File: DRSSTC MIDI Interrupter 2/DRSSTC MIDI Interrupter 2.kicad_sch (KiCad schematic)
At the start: 67 parts, among them CN2 HX25003-2WAP, Q1 8205A_C5370944, Q2 AO3401A_C347476, SW1 SW_Push, SW2 SW_Push, U1 ESP32-S3-WROOM-1, U10 TPS63802DLAR, U11 BQ27441DRZR-G1B, U2 BQ24072RGT, U3 DW01A, U4 TPS61023DRLR, U6 SRV05-4, U7 USBLC6-2P6, U8 TS3USB221ARSER, U9 TL331

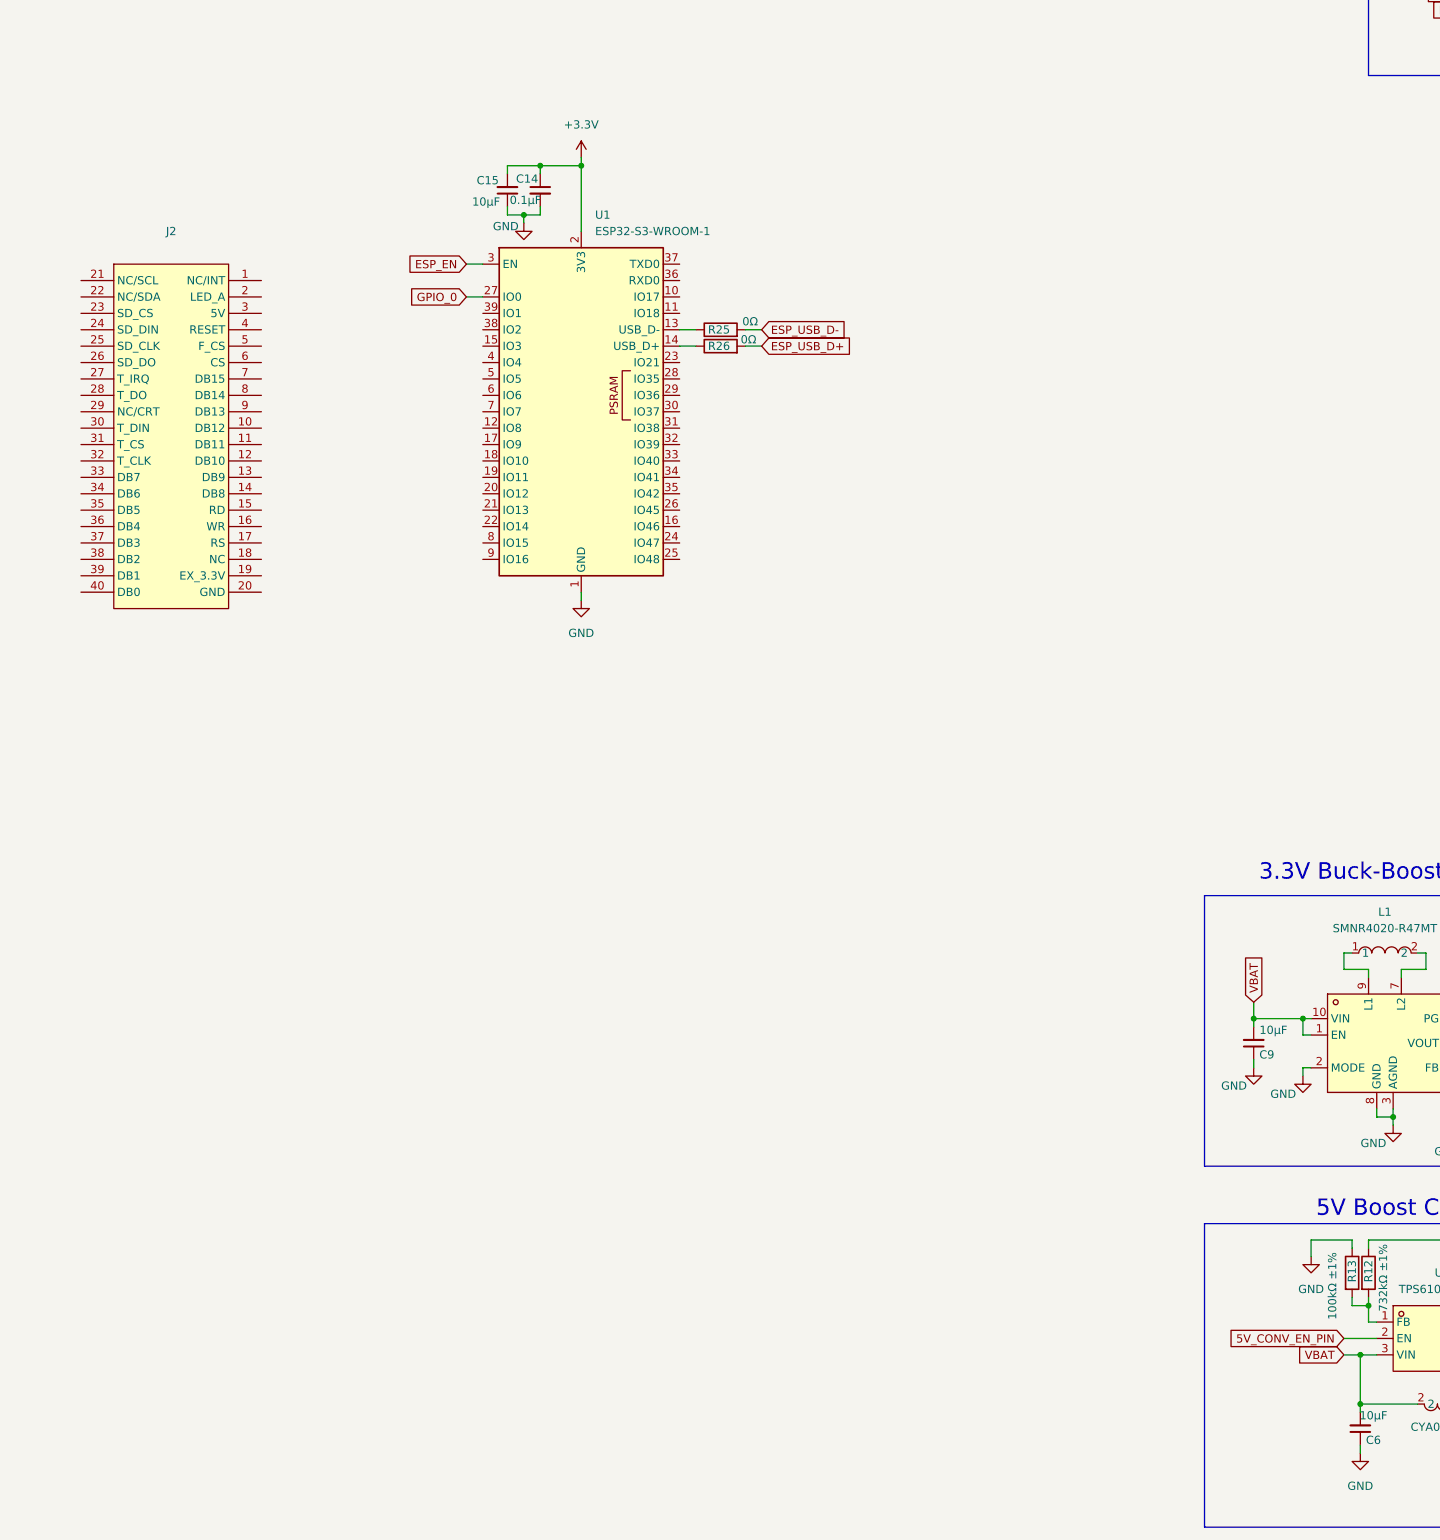
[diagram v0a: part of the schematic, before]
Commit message: Initial commit of components
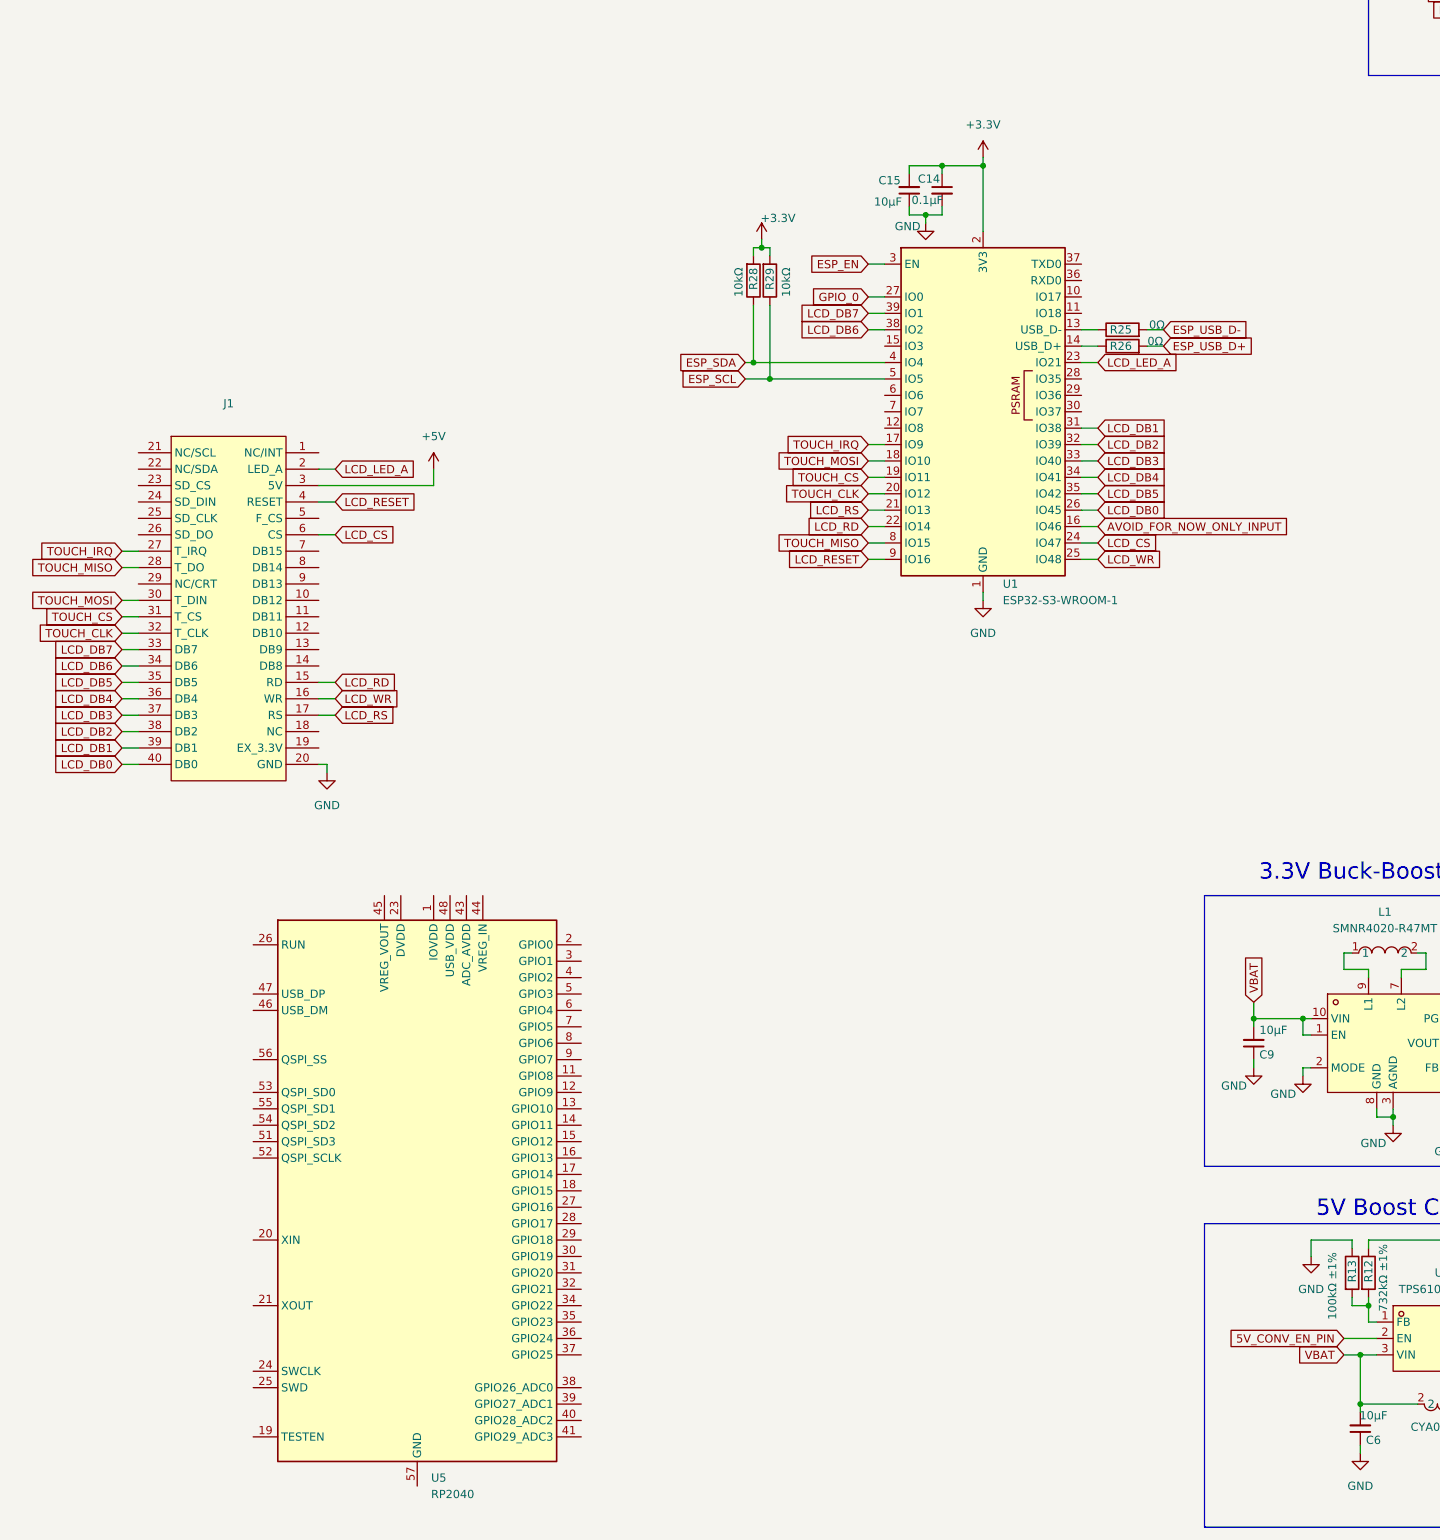
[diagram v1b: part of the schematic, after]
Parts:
- removed J2: ~, Custom Parts:LCD, symbol Custom Parts:LCD
- added J1: ~, parts:LCD, symbol parts:LCD
- added R28, R29: 10kΩ, Resistor_SMD:R_0805_2012Metric_Pad1.20x1.40mm_HandSolder, symbol Device:R
- added U5: RP2040, Package_DFN_QFN:QFN-56-1EP_7x7mm_P0.4mm_EP3.2x3.2mm, symbol MCU_RaspberryPi:RP2040
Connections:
- net +3.3V: now also R28.2, R29.2
- net +5V: now also J1.3 (5V)
- net ESP_SCL: now also U1.5 (IO5), R29.1
- net ESP_SDA: now also U1.4 (IO4), R28.1
- net GND: now also J1.20 (GND)
- net AVOID_FOR_NOW_ONLY_INPUT: now reaches U1.16 (IO46)
- net TOUCH_IRQ: now reaches U1.17 (IO9)
- net TOUCH_IRQ: now also J1.27 (T_IRQ)
- net TOUCH_MOSI: now reaches U1.18 (IO10)
- net TOUCH_MOSI: now also J1.30 (T_DIN)
- net TOUCH_CS: now reaches U1.19 (IO11)
- net TOUCH_CS: now also J1.31 (T_CS)
- net TOUCH_CLK: now reaches U1.20 (IO12)
- net TOUCH_CLK: now also J1.32 (T_CLK)
- net LCD_RS: now reaches U1.21 (IO13)
- net LCD_RS: now also J1.17 (RS)
- net LCD_RD: now reaches U1.22 (IO14)
- net LCD_RD: now also J1.15 (RD)
- net LCD_LED_A: now reaches U1.23 (IO21)
- net LCD_LED_A: now also J1.2 (LED_A)
- net LCD_CS: now reaches U1.24 (IO47)
- net LCD_CS: now also J1.6 (CS)
- net LCD_WR: now reaches U1.25 (IO48)
- net LCD_WR: now also J1.16 (WR)
- net LCD_DB0: now reaches U1.26 (IO45)
- net LCD_DB0: now also J1.40 (DB0)
- net LCD_DB1: now reaches U1.31 (IO38)
- net LCD_DB1: now also J1.39 (DB1)
- net LCD_DB2: now reaches U1.32 (IO39)
- net LCD_DB2: now also J1.38 (DB2)
- net LCD_DB3: now reaches U1.33 (IO40)
- net LCD_DB3: now also J1.37 (DB3)
- net LCD_DB4: now reaches U1.34 (IO41)
- net LCD_DB4: now also J1.36 (DB4)
- net LCD_DB5: now reaches U1.35 (IO42)
- net LCD_DB5: now also J1.35 (DB5)
- net LCD_DB6: now reaches U1.38 (IO2)
- net LCD_DB6: now also J1.34 (DB6)
- net LCD_DB7: now reaches U1.39 (IO1)
- net LCD_DB7: now also J1.33 (DB7)
- net TOUCH_MISO: now reaches U1.8 (IO15)
- net TOUCH_MISO: now also J1.28 (T_DO)
- net LCD_RESET: now reaches U1.9 (IO16)
- net LCD_RESET: now also J1.4 (RESET)
- new net: U5.1 (IOVDD), U5.10 (IOVDD), U5.22 (IOVDD), U5.33 (IOVDD), U5.42 (IOVDD), U5.49 (IOVDD)
- new net: U5.23 (DVDD), U5.50 (DVDD)
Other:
- moved on the sheet: C14, C15, R25, R26, U1
